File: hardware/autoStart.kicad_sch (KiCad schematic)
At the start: 22 parts, among them J1 AudioJack3_Switch, J2 Screw_Terminal_01x03, Q1 BC547, U1 ICL7621BMTV, U2 ICL7621BMTV, U3 78S05M

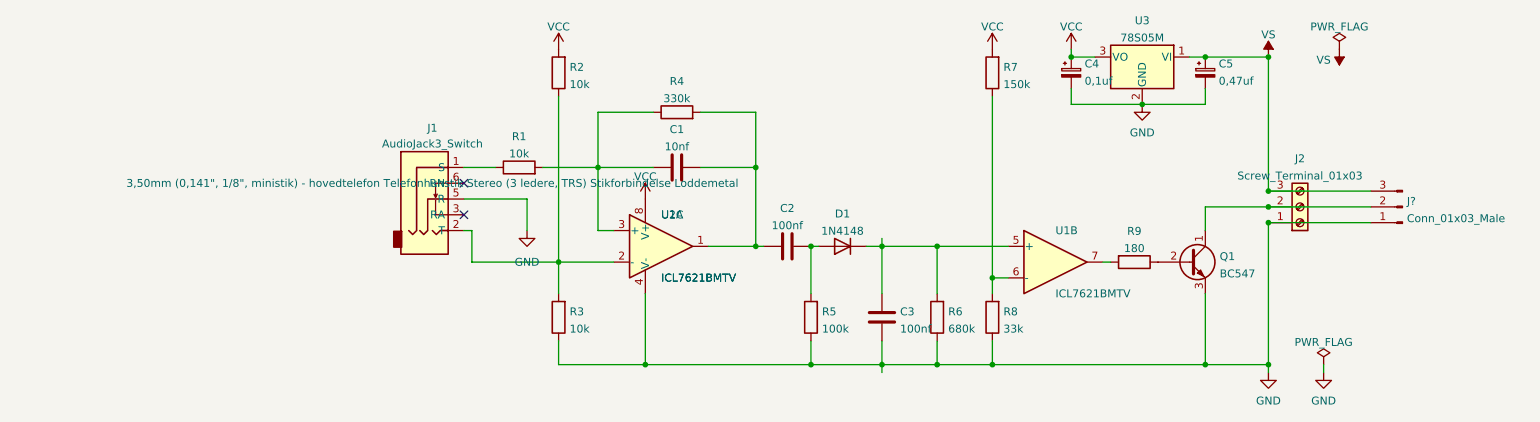
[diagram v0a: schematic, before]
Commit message: SMD Mounts Initial commit
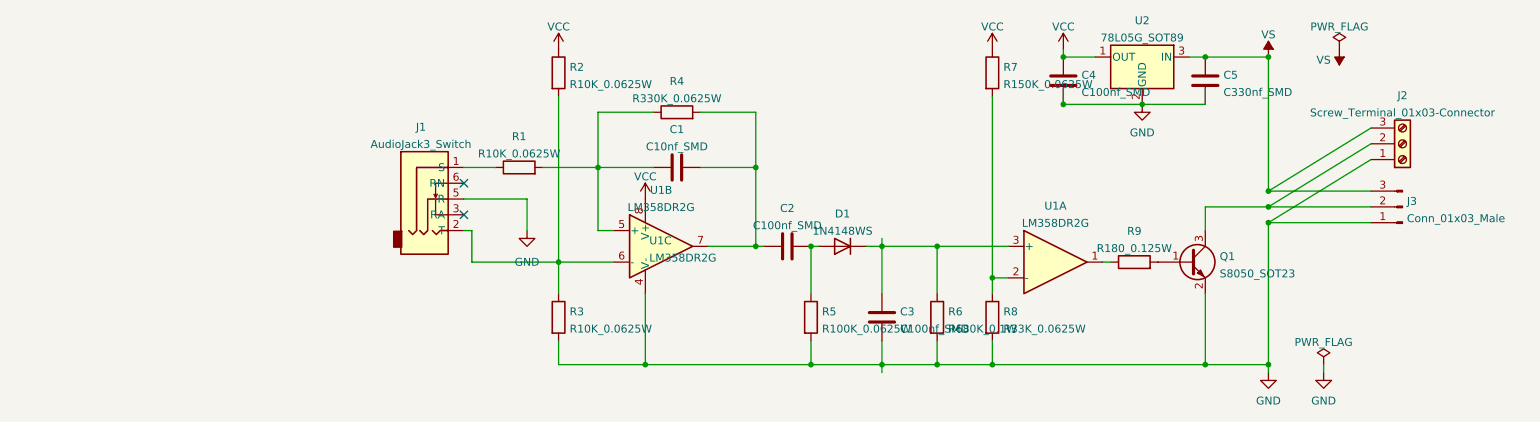
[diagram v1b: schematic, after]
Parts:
- removed C1: 10nf, Capacitor_THT:C_Disc_D4.3mm_W1.9mm_P5.00mm, symbol Device:C
- removed C2, C3: 100nf, Capacitor_THT:C_Disc_D3.8mm_W2.6mm_P2.50mm, symbol Device:C
- removed C4: 0,1uf, Capacitor_THT:CP_Radial_Tantal_D5.0mm_P5.00mm, symbol Device:C_Polarized_Small
- removed C5: 0,47uf, Capacitor_THT:CP_Radial_Tantal_D5.0mm_P5.00mm, symbol Device:C_Polarized_Small
- removed D1: 1N4148, Diode_THT:D_DO-35_SOD27_P7.62mm_Horizontal, symbol Diode:1N4148
- removed J2: Screw_Terminal_01x03, TerminalBlock_Phoenix:TerminalBlock_Phoenix_MKDS-1,5-3_1x03_P5.00mm_Horizontal, symbol Connector:Screw_Terminal_01x03
- removed J?: Conn_01x03_Male, symbol Connector:Conn_01x03_Male
- removed Q1: BC547, Package_TO_SOT_THT:TO-92L_Inline_Wide, symbol Transistor_BJT:BC547
- removed R1, R2, R3: 10k, Resistor_THT:R_Axial_DIN0411_L9.9mm_D3.6mm_P12.70mm_Horizontal, symbol Device:R
- removed R4: 330k, Resistor_THT:R_Axial_DIN0411_L9.9mm_D3.6mm_P12.70mm_Horizontal, symbol Device:R
- removed R5: 100k, Resistor_THT:R_Axial_DIN0411_L9.9mm_D3.6mm_P12.70mm_Horizontal, symbol Device:R
- removed R6: 680k, Resistor_THT:R_Axial_DIN0411_L9.9mm_D3.6mm_P12.70mm_Horizontal, symbol Device:R
- removed R7: 150k, Resistor_THT:R_Axial_DIN0411_L9.9mm_D3.6mm_P12.70mm_Horizontal, symbol Device:R
- removed R8: 33k, Resistor_THT:R_Axial_DIN0411_L9.9mm_D3.6mm_P12.70mm_Horizontal, symbol Device:R
- removed R9: 180, Resistor_THT:R_Axial_DIN0411_L9.9mm_D3.6mm_P12.70mm_Horizontal, symbol Device:R
- removed U1, U2: ICL7621BMTV, Package_TO_SOT_THT:TO-99-8, symbol Local_Miscellaneous_Library:ICL7621BMTV
- removed U3: 78S05M, Package_TO_SOT_SMD:SOT-89-3, symbol Regulator_Linear:LM7805_TO220
- added C1: C10nf_SMD, Capacitor_SMD:C_0402_1005Metric, symbol Local_Device_Library:C10nf_SMD
- added C2, C3, C4: C100nf_SMD, Capacitor_SMD:C_0402_1005Metric, symbol Local_Device_Library:C100nf_SMD
- added C5: C330nf_SMD, Capacitor_SMD:C_0805_2012Metric, symbol Local_Device_Library:C330nf_SMD
- added D1: 1N4148WS, Diode_SMD:D_SOD-323F, symbol Local_Diode_Library:1N4148WS
- added J2: Screw_Terminal_01x03-Connector, Local_Connectors:Phoenix_TERM_BLOCK_3POS_45DEG_5MM_PCB, symbol Local_Connectors_Library:Screw_Terminal_01x03-Connector
- added J3: Conn_01x03_Male, Local_Project_Connectors_Library:PinHeader_1x03_P_5mm_Vertical-(Backside_Mount), symbol Connector:Conn_01x03_Male
- added Q1: S8050_SOT23, Package_TO_SOT_SMD:SOT-23, symbol Local_Transistor_BJT_Library:S8050_SOT23
- added R1, R2, R3: R10K_0.0625W, Resistor_SMD:R_0402_1005Metric, symbol Local_Device_Library:R10K_0.0625W
- added R4: R330K_0.0625W, Resistor_SMD:R_0402_1005Metric, symbol Local_Device_Library:R330K_0.0625W
- added R5: R100K_0.0625W, Resistor_SMD:R_0402_1005Metric, symbol Local_Device_Library:R100K_0.0625W
- added R6: R680K_0.1W, Resistor_SMD:R_0201_0603Metric, symbol Local_Device_Library:R680K_0.1W
- added R7: R150K_0.0625W, Resistor_SMD:R_0402_1005Metric, symbol Local_Device_Library:R150K_0.0625W
- added R8: R33K_0.0625W, Resistor_SMD:R_0402_1005Metric, symbol Local_Device_Library:R33K_0.0625W
- added R9: R180_0.125W, Resistor_SMD:R_0805_2012Metric, symbol Local_Device_Library:R180_0.125W
- added U1: LM358DR2G, Package_SO:SOIC-8_3.9x4.9mm_P1.27mm, symbol Local_Miscellaneous_Library:LM358DR2G
- added U2: 78L05G_SOT89, Package_TO_SOT_SMD:SOT-89-3, symbol Local_Miscellaneous_Library:78L05G_SOT89
- J1: footprint Local_Connectors:AUDIO_JACK_ASJ-195-L-HT -> Local_Connectors:AUDIO_JACK_ASJ-195-L-HT-(Backside_Mount)
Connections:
- net GND: now also C3.2, C4.2, C5.2, J2.1 (Pin_1), J3.1 (Pin_1), Q1.2 (E), R3.2, R5.2, R6.2, R8.2, U1.4 (V-), U2.2 (GND)
- net VCC: now also C4.1, R2.1, R7.1, U1.8 (V+), U2.1 (OUT)
- net VS: now also C5.1, J2.3 (Pin_3), J3.3 (Pin_3), U2.3 (IN)
- net at J1.2 (T): now also R2.2, R3.1, U1.6 (-)
- net at J1.1 (S): now also R1.1
- new net: C1.1, R1.2, R4.1, U1.5 (+)
- new net: C1.2, C2.1, R4.2, U1.7
- new net: C2.2, D1.2 (A), R5.1
- new net: R7.2, R8.1, U1.2 (-)
- new net: J2.2 (Pin_2), J3.2 (Pin_2), Q1.3 (C)
- new net: C3.1, D1.1 (K), R6.1, U1.3 (+)
- new net: Q1.1 (B), R9.2
- new net: R9.1, U1.1
